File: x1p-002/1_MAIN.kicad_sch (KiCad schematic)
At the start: 57 parts, among them P1 A_A4, U2 FT2232HL, U3 TPS54202DDCR, U4 LM1084S-3.3/TR, X2 12MHz

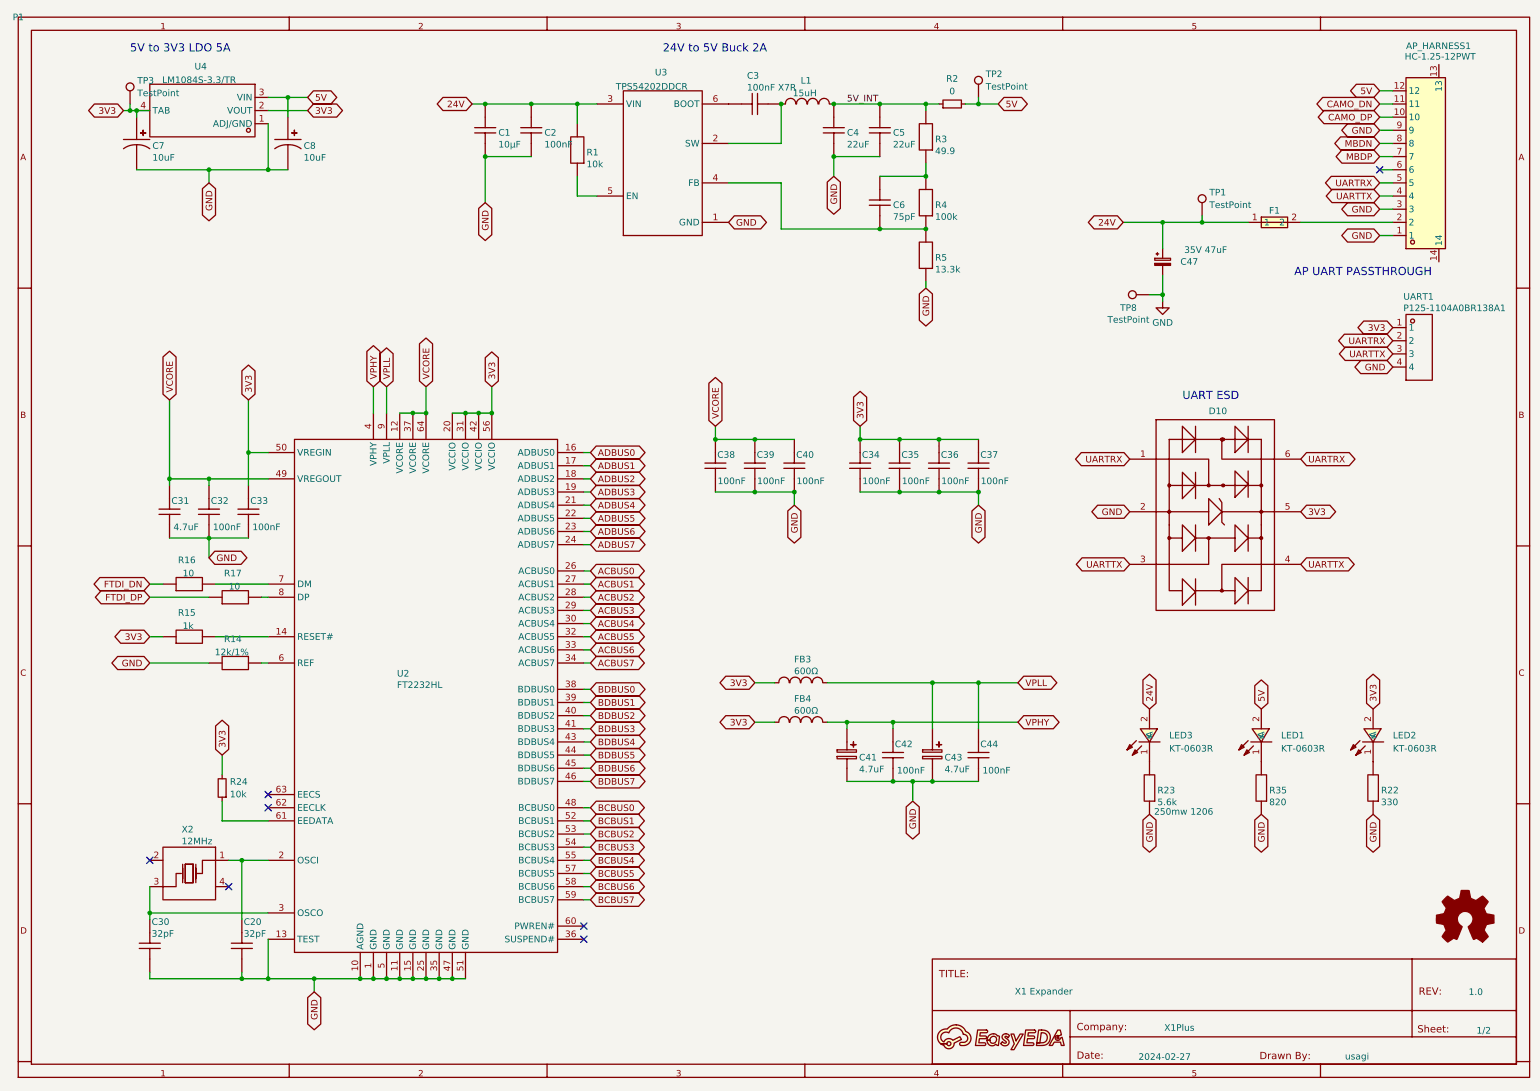
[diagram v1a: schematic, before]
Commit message: X1P-002: schematic: redesign with larger 5V buck (#60), add 3V3 buck (#63), add OCP circuits for 3V3 and 5V (but not connected to user ports yet; #61)
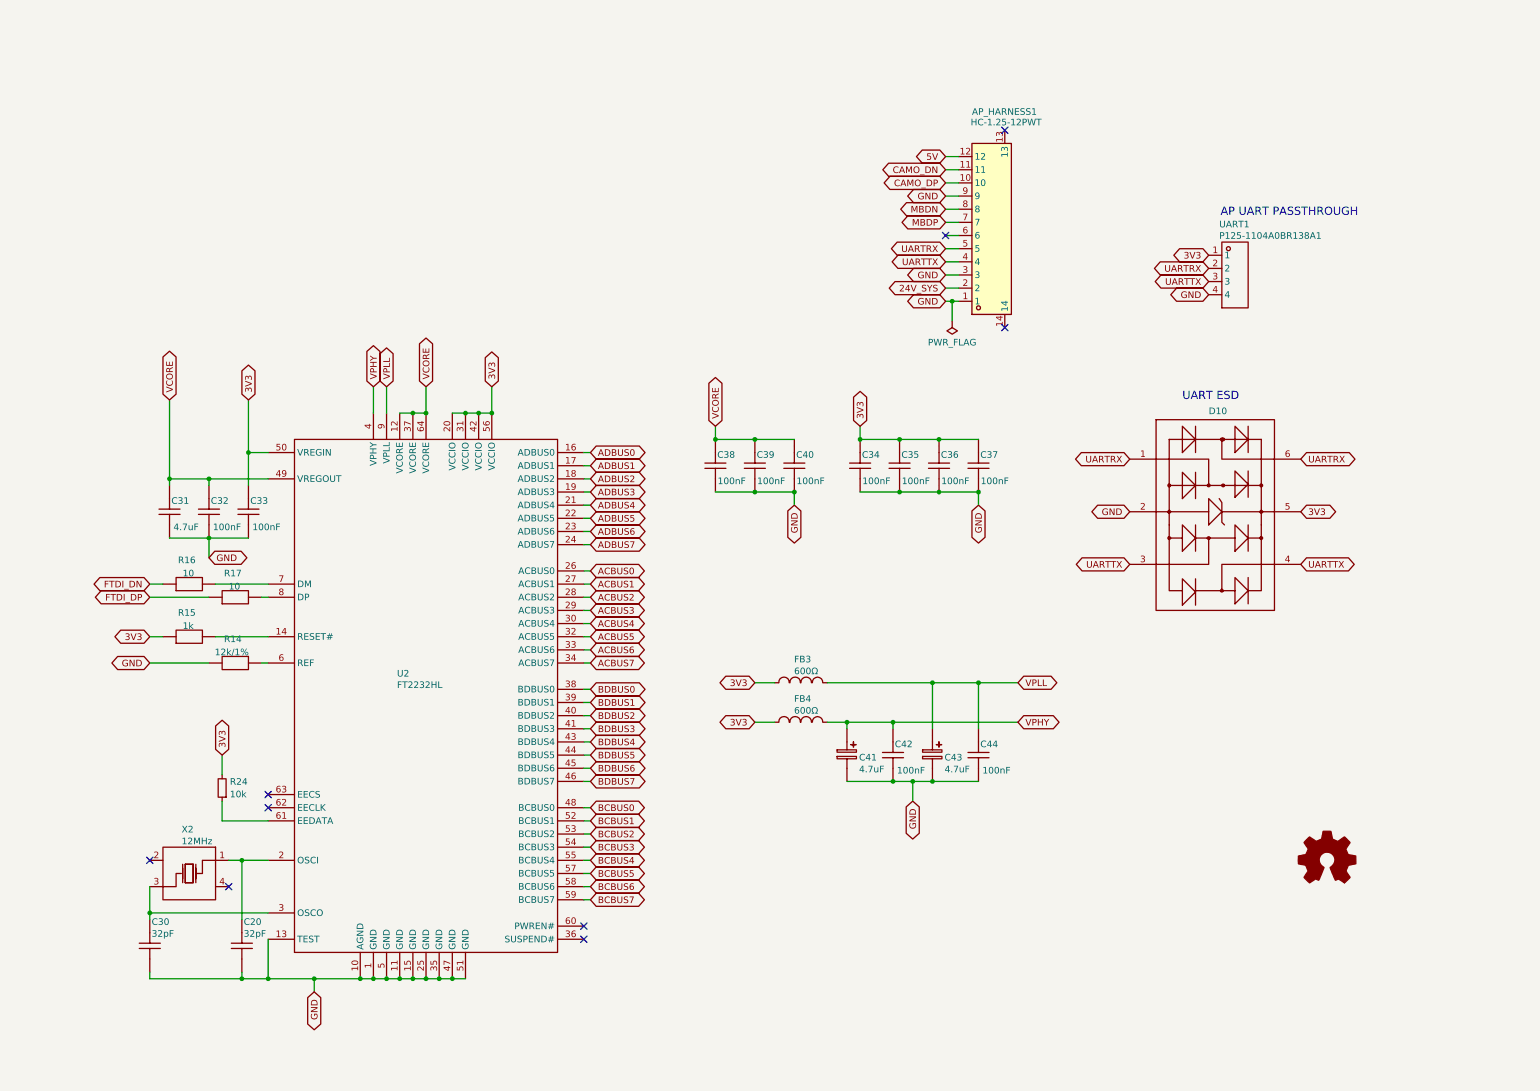
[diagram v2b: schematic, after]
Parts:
- removed C1: 10µF, Capacitor_SMD:C_0805_2012Metric, symbol x1-expander:100nF
- removed C2: 100nF, Capacitor_SMD:C_0603_1608Metric, symbol x1-expander:100nF
- removed C3: 100nF X7R, Capacitor_SMD:C_0603_1608Metric, symbol x1-expander:100nF
- removed C4, C5: 22uF, Capacitor_SMD:C_0603_1608Metric, symbol x1-expander:22uF
- removed C47: 35V 47uF, Capacitor_SMD:CP_Elec_6.3x5.8, symbol Device:C_Polarized_Small
- removed C6: 75pF, Capacitor_SMD:C_0603_1608Metric, symbol x1-expander:75pF
- removed C7, C8: 10uF, Capacitor_SMD:C_0805_2012Metric, symbol x1-expander:10uF
- removed F1: BSMD1206-100-30V, x1-expander:F1206, symbol x1-expander:BSMD1206-100-30V
- removed L1: 15uH, x1-expander:IND-SMD_L7.2-W6.6_GPSR07X0, symbol x1-expander:15uH
- removed LED1, LED2, LED3: KT-0603R, x1-expander:LED0603-RD, symbol x1-expander:KT-0603R
- removed P1: A_A4, x1-expander:, symbol x1-expander:A_A4
- removed R1: 10k, Resistor_SMD:R_0603_1608Metric, symbol x1-expander:511k
- removed R2: 0, Resistor_SMD:R_0603_1608Metric, symbol Device:R_Small
- removed R22: 330, Resistor_SMD:R_0603_1608Metric, symbol x1-expander:10kΩ
- removed R23: 5.6k, Resistor_SMD:R_1206_3216Metric, symbol x1-expander:10kΩ
- removed R3: 49.9, Resistor_SMD:R_0603_1608Metric, symbol x1-expander:49.9
- removed R35: 820, Resistor_SMD:R_0603_1608Metric, symbol x1-expander:10kΩ
- removed R4: 100k, Resistor_SMD:R_0603_1608Metric, symbol x1-expander:100k
- removed R5: 13.3k, Resistor_SMD:R_0603_1608Metric, symbol x1-expander:13.3k
- removed TP1, TP2, TP3, TP8: TestPoint, TestPoint:TestPoint_Pad_D1.0mm, symbol Connector:TestPoint
- removed U3: TPS54202DDCR, x1-expander:SOT-23-6_L2.9-W1.6-P0.95-LS2.8-BL-2, symbol x1-expander:TPS54202DDCR
- removed U4: LM1084S-3.3/TR, x1-expander:TO-263-3_L8.6-W10.2-P2.54-LS14.4-TL, symbol x1-expander:LM1084S-3.3/TR
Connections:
- net 24V_SYS: now reaches AP_HARNESS1.2
- no-connect marks 7 -> 9
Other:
- note removed: "24V to 5V Buck 2A"
- note removed: "5V to 3V3 LDO 5A"
- title: (none) -> X1Plus Expansion Board: X1P-002
- moved on the sheet: AP_HARNESS1, UART1
